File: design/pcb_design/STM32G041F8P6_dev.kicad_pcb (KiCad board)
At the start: 4 copper layers, 70 x 50 mm, 45 parts, among them J1 USB_B_Micro, J2 S2B-PH-K-S, J3 Conn_02x02_Odd_Even, J4 Conn_ST_STDC14, SW1 Reset, SW2 Up, SW3 Enter, SW4 Down, U1 MCP73831-2-OT, U2 MIC5301-3.3YD5, U3 STM32G041F8Px, U4 ADXL343BCCZ, Y1 Crystal

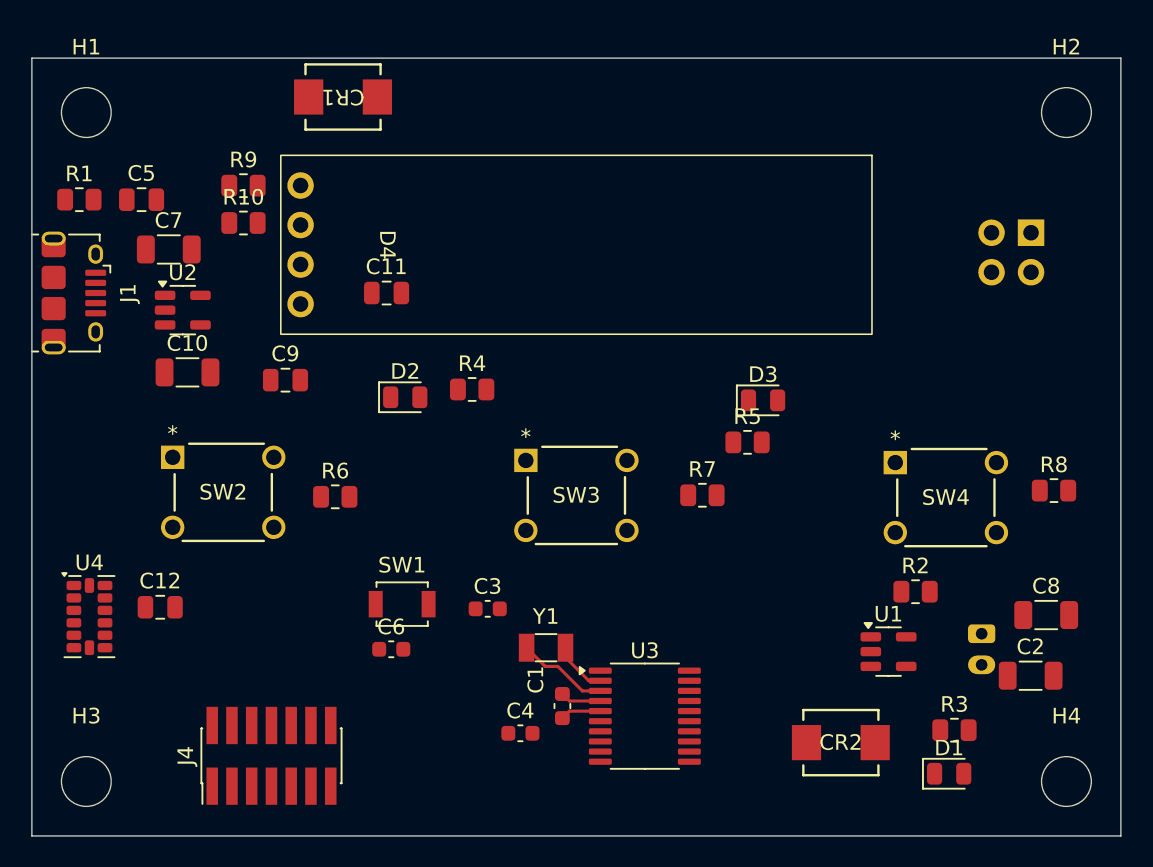
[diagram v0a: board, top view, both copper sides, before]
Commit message: pcb updates
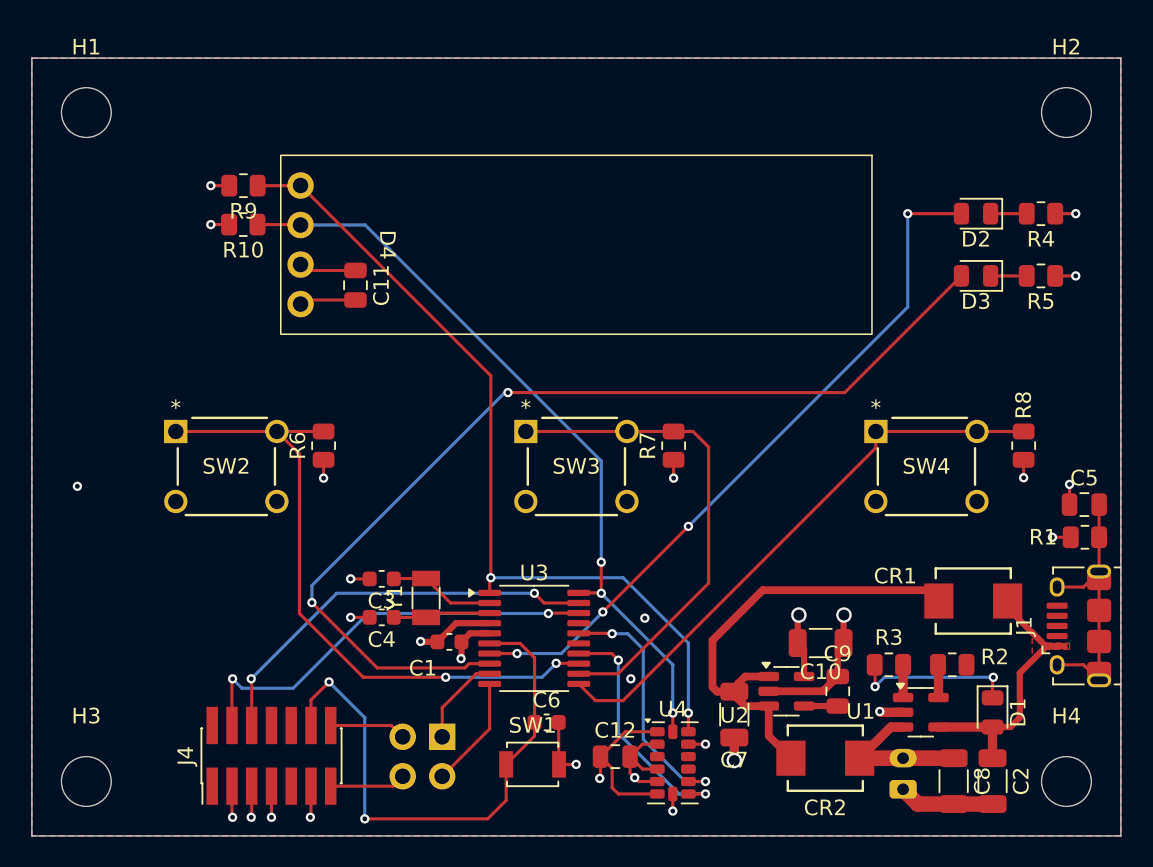
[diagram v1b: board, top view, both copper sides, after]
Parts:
- moved R1 68.2 mm to (223.7, 76.8), turned to 180 degrees
- moved J1 68.1 mm to (223.3, 82.5), turned to 90 degrees
- moved C5 63.7 mm to (223.7, 74.7), turned to 180 degrees
- moved CR1 51.9 mm to (216.5, 80.9), turned to 0 degrees
- moved J3 49.8 mm to (182.4, 89.6)
- moved C7 47.1 mm to (201.2, 88.2), turned to 90 degrees
- moved U2 45.9 mm to (204.5, 86.7)
- moved C10 44.3 mm to (206.7, 83.6), turned to 180 degrees
- moved C9 40.7 mm to (207.8, 86.7), turned to 90 degrees
- moved U4 38.7 mm to (197.2, 91.3)
- moved D2 38.5 mm to (216.7, 56.0), turned to 180 degrees
- moved R4 38.3 mm to (220.9, 56.0), turned to 180 degrees
- moved C12 30.8 mm to (193.5, 90.9)
- moved R5 21.7 mm to (220.9, 60.0), turned to 180 degrees
- moved D3 15.9 mm to (216.7, 60.0), turned to 180 degrees
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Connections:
- C8 pad 1: Net-(J2-Pin_2) -> +BATT
- J2 pad 2: Net-(J2-Pin_2) -> +BATT
- SW2 pad 3: +3V3 -> +3.3V
- SW2 pad 4: +3V3 -> +3.3V
- SW3 pad 3: +3V3 -> +3.3V
- SW3 pad 4: +3V3 -> +3.3V
- SW4 pad 3: +3V3 -> +3.3V
- SW4 pad 4: +3V3 -> +3.3V
- U1 pad 3: Net-(J2-Pin_2) -> +BATT
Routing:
- net /PA1: track 0.00 -> 64.4 mm, vias 0 -> 2
- net SDA: track 0.00 -> 54.2 mm, vias 0 -> 2
- net GND: track 2.62 -> 54.1 mm, vias 0 -> 22
- net SCL: track 0.00 -> 49.2 mm, vias 0 -> 3
- net /PA0: track 0.00 -> 45.6 mm, vias 0 -> 4
- net /PA6: track 0.00 -> 41.8 mm, vias 0 -> 2
- net /PA4: track 0.00 -> 36.8 mm
- net Net-(J4-~{RST}): track 0.00 -> 35.8 mm, vias 0 -> 2
- net /PA5: track 0.00 -> 31.7 mm
- net Net-(U2-EN): track 0.00 -> 29.9 mm
- net /SWDIO: track 0.00 -> 27.5 mm, vias 0 -> 2
- net +3.3V: track 2.62 -> 29.4 mm, vias 0 -> 7
- net /SWCLK: track 0.00 -> 26.6 mm, vias 0 -> 2
- net VBUS: track 0.00 -> 18.1 mm
- net Net-(J1-Shield): track 0.00 -> 17.1 mm
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- added copper zone on In2.Cu, net +3.3V
- added copper zone on B.Cu, net GND
- added copper zone on F.Cu, net GND
- added copper zone on In1.Cu, net GND
- added copper zone on F.Cu, net VBUS
